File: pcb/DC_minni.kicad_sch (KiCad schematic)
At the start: 56 parts, among them J1 DRUCKSENSOR, J2 Encoder, U1 ESP32-DevKitC, U2 USB-C to DIP PCB

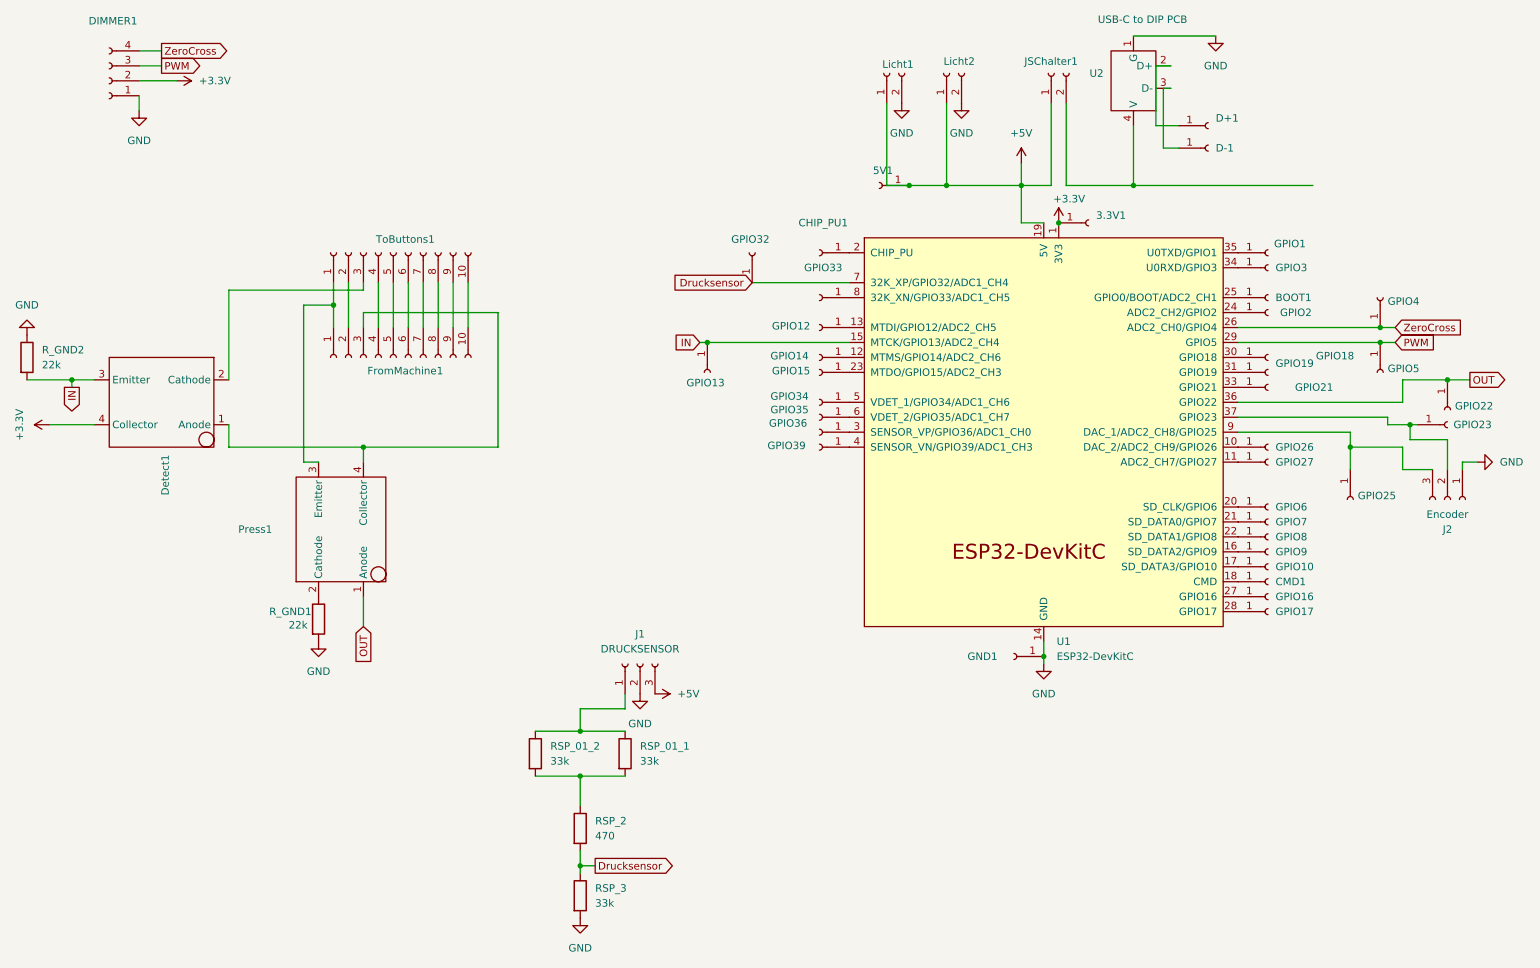
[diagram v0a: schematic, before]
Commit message: Combining main and old main with claude
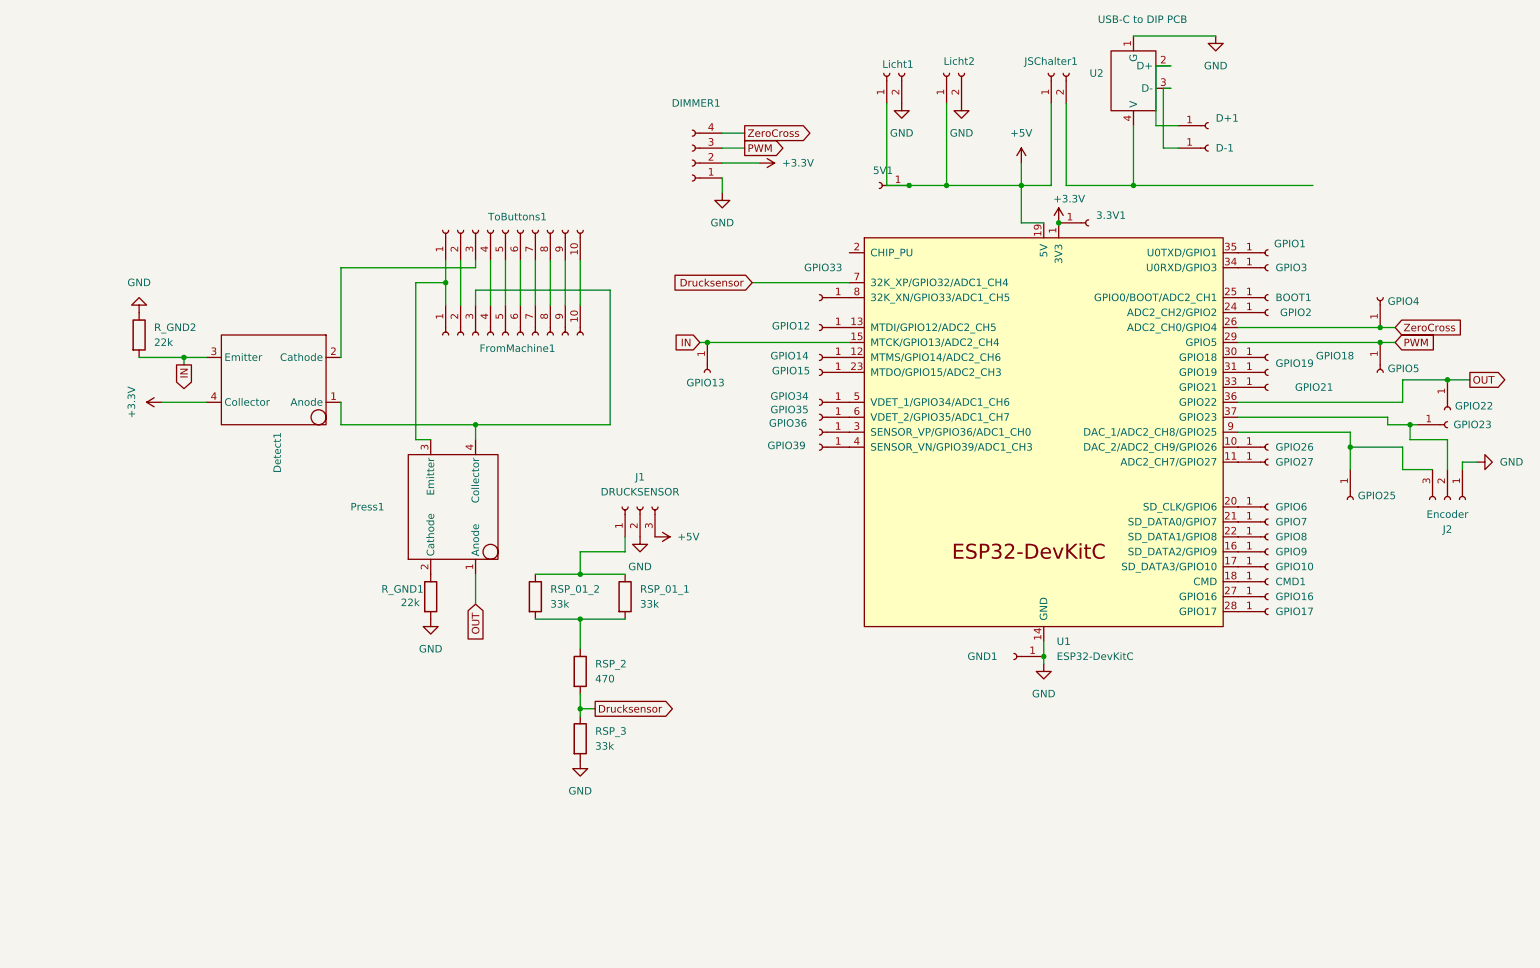
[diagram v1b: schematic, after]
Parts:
- removed CHIP_PU1, GPIO32: Conn_01x01_Socket, Connector_PinHeader_2.54mm:PinHeader_1x01_P2.54mm_Vertical, symbol Connector:Conn_01x01_Socket
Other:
- moved on the sheet: DIMMER1, Detect1, FromMachine1, J1, Press1, RSP_01_1, RSP_01_2, RSP_2, RSP_3, R_GND1, R_GND2, ToButtons1
